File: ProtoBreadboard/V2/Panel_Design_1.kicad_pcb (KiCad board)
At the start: 2 copper layers, 121.8 x 57.9 mm, 146 parts, among them J13 Conn_01x08_Female, J14 Conn_01x08_Female, J18 Conn_01x07_Female, J2 Conn_01x10_Female, J25 Conn_01x07_Female, J33 Conn_01x10_Female, J34 Conn_01x10_Female, J35 Conn_01x10_Female, J36 Conn_01x10_Female, J37 Conn_01x10_Female, J38 Conn_01x10_Female, J39 Conn_01x10_Female, J4 Conn_01x10_Female, J40 Conn_01x10_Female, J41 Conn_01x10_Female, J42 Conn_01x10_Female, J43 Conn_01x10_Female, J44 Conn_01x10_Female, J45 Conn_01x10_Female, J46 Conn_01x10_Female, J47 Conn_01x10_Female, J48 Conn_01x10_Female, J49 Conn_01x10_Female, J50 Conn_01x10_Female

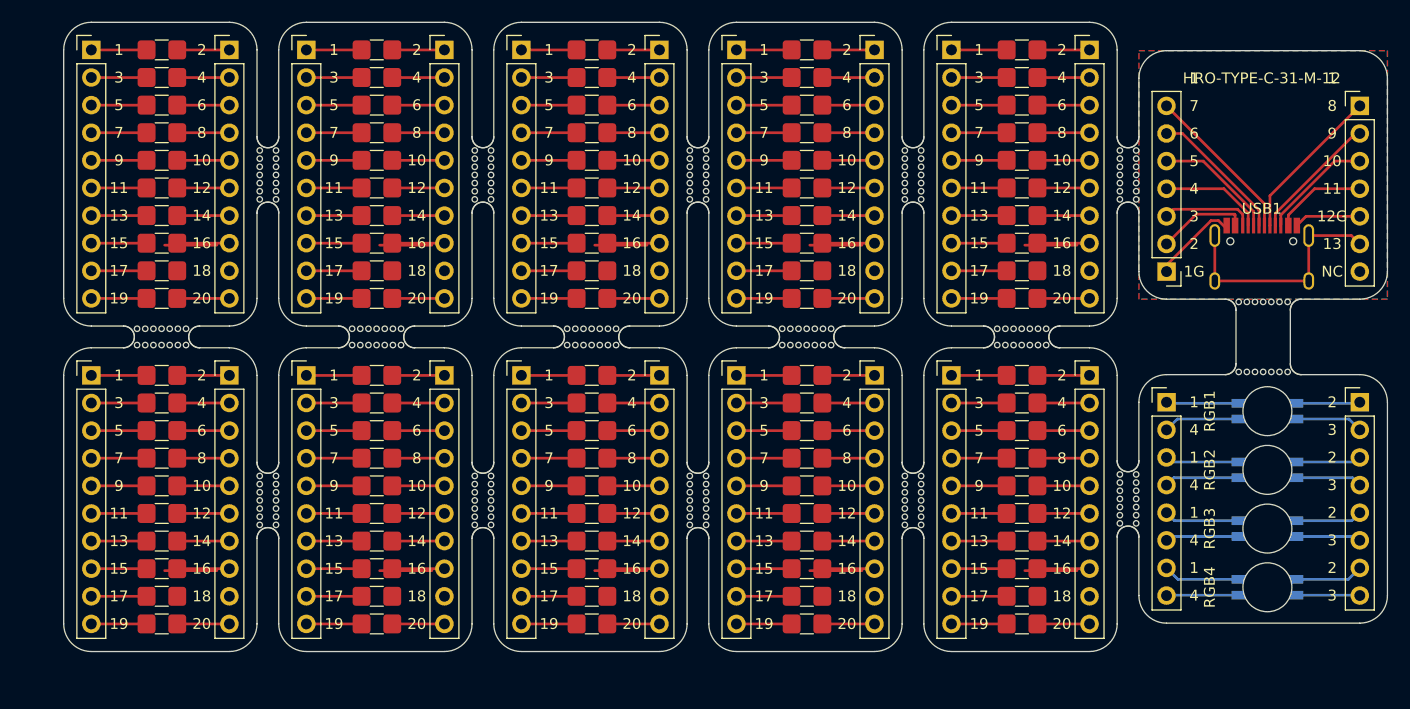
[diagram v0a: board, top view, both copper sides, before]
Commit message: Added Gerber Files for all 3 new designs
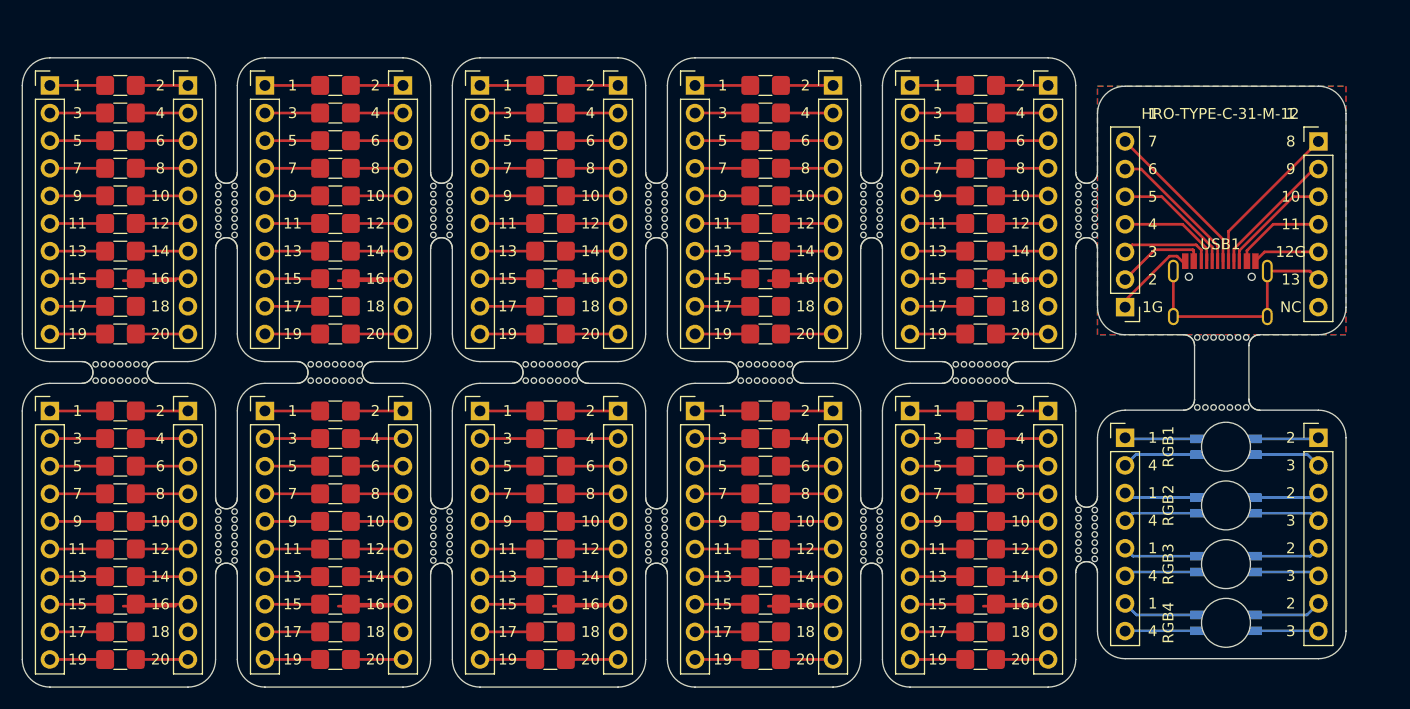
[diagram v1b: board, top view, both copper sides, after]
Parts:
- moved J13 5.02 mm to (124.3, 55.8)
- moved G100 5.02 mm to (111.0, 76.2)
- moved G76 5.02 mm to (71.4, 66.0)
- moved G78 5.02 mm to (71.4, 71.1)
- moved G80 5.02 mm to (71.4, 76.2)
- moved G86 5.02 mm to (91.2, 66.0)
- moved G88 5.02 mm to (91.2, 71.1)
- moved G90 5.02 mm to (91.2, 76.2)
- moved G96 5.02 mm to (111.0, 66.0)
- moved G98 5.02 mm to (111.0, 71.1)
- moved G22 5.02 mm to (71.4, 25.9)
- moved G23 5.02 mm to (71.4, 28.5)
- moved G24 5.02 mm to (71.4, 31.0)
- moved G25 5.02 mm to (71.4, 33.6)
- moved G26 5.02 mm to (71.4, 36.1)
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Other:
- outline, holes or cut-outs redrawn
